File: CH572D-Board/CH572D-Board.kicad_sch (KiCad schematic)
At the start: 6 parts, among them J1 Conn_PinHeader_1x08_P2.54mm_V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, J2 Conn_PinHeader_2x02_P1.27mm_V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, Y1 32mhz

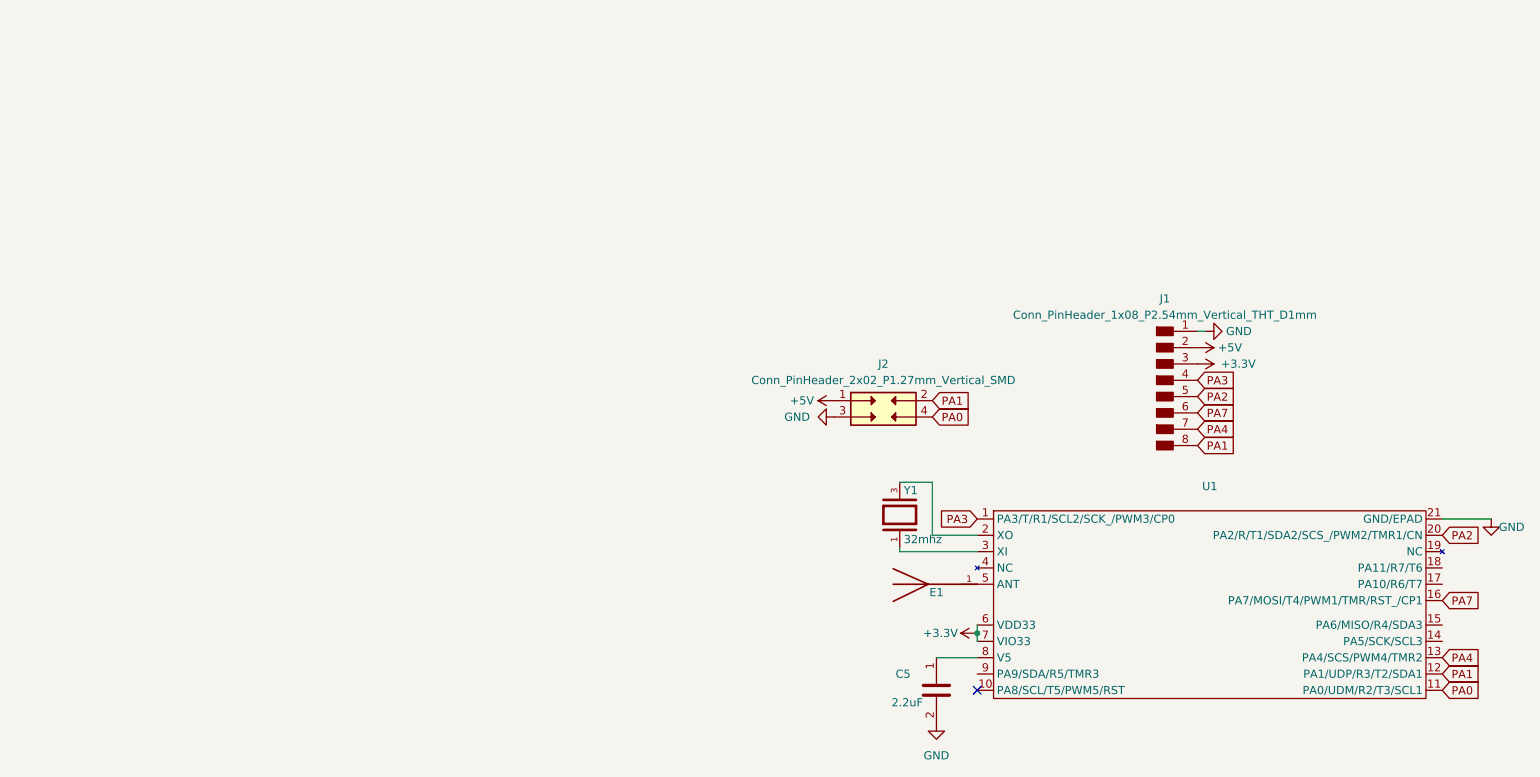
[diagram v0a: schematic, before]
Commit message: small work mostlty useless
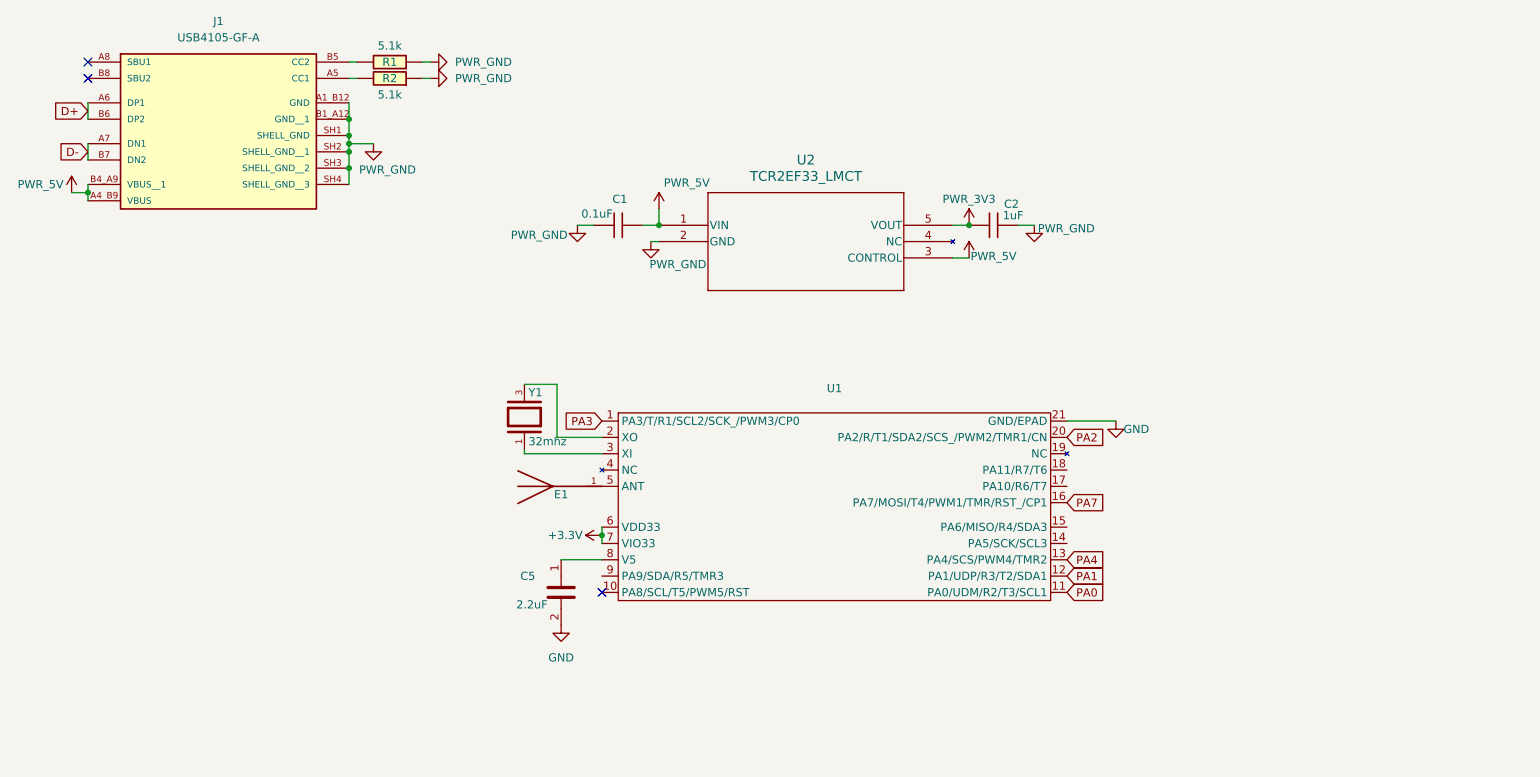
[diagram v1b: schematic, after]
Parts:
- removed J1: Conn_PinHeader_1x08_P2.54mm_Vertical_THT_D1mm, fab:PinHeader_1x08_P2.54mm_Vertical_THT_D1mm, symbol fab:Conn_PinHeader_1x08_P2.54mm_Vertical_THT_D1mm
- removed J2: Conn_PinHeader_2x02_P1.27mm_Vertical_SMD, fab:PinSocket_1x04_P2.54mm_Vertical_SMD, symbol fab:Conn_PinHeader_2x02_P1.27mm_Vertical_SMD
- added C1: 0.1uF, fab:C_0603, symbol fab:C_0603
- added C2: 1uF, fab:C_0603, symbol fab:C_0603
- added J1: USB4105-GF-A, USB4105-GF-A:GCT_USB4105-GF-A, symbol usbc:USB4105-GF-A
- added R1, R2: 5.1k, fab:R_0603, symbol fab:R_0603
- added U2: TCR2EF33_LMCT, Footprint:voltage regulator, symbol voltage regulator:TCR2EF33_LMCT
- C5: footprint Personal:0603 -> Footprint:0603
- E1: footprint Personal:pcbantenna -> Footprint:pcbantenna
- U1: footprint Ch572D:CH572D -> Footprint:CH572D
- Y1: footprint Personal:32mhz crystal -> Footprint:32mhz crystal
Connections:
- new net: J1.A5 (CC1), R2.1
- new net: J1.B5 (CC2), R1.1
- new net D+: J1.A6 (DP1), J1.B6 (DP2)
- new net D-: J1.A7 (DN1), J1.B7 (DN2)
- new net PWR_3V3: C2.1, U2.5 (VOUT)
- new net PWR_5V: C1.2, J1.A4_B9 (VBUS), J1.B4_A9 (VBUS__1), U2.1 (VIN), U2.3 (CONTROL)
- new net PWR_GND: C1.1, C2.2, J1.A1_B12 (GND), J1.B1_A12 (GND__1), J1.SH1 (SHELL_GND), J1.SH2 (SHELL_GND__1), J1.SH3 (SHELL_GND__2), J1.SH4 (SHELL_GND__3), R1.2, R2.2, U2.2 (GND)
- no-connect marks 1 -> 3
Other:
- moved on the sheet: C5, E1, U1, Y1
